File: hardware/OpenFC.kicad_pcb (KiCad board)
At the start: 6 copper layers, 27.6 x 27.6 mm, 135 parts, among them J10 5V, J12 5V, J14 5V, J15 5V, J17 5V, J18 5V, J20 5V, J21 5V, J22 5V, J24 5V, J25 5V, J26 5V, J27 5V, J28 5V, J29 5V, J30 5V, J31 5V, J32 5V, J33 5V, J34 5V, J35 5V, J37 5V, J39 5V, J40 5V, J41 5V, J42 5V, J43 5V, J44 5V, J45 5V, J46 5V, J48 5V, J49 5V, J5 5V, J8 5V, P1 SM08B-SRSS-TB(LF)(SN), Q5 AP1606, Q6 AP1606, U1 COS8051SOT, U10 RP2354A, U11 TS2306A 240GF MSM 9_C2976675, U18 SN74LVC1G3157DTBR, U2 TLV7031DPWR, U3 TI LMR51430YFDDCR, U4 TI LMR51430YFDDCR, U5 TPS2116DRLR, U6 NCV8187AMT180TAG, U7 LP5912-3.3DRVR, U8 SM06B-SRSS-TB(LF)(SN), U9 LSM6DSV16XTR, X1 XTM25012000JT00351001

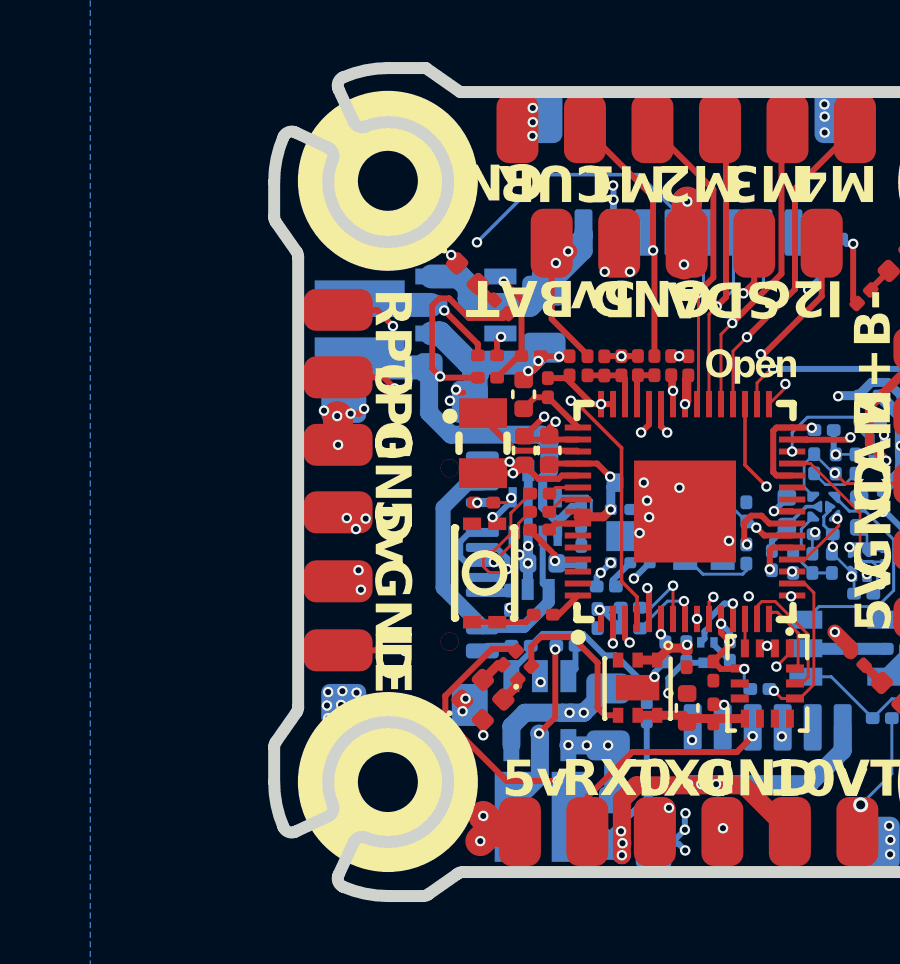
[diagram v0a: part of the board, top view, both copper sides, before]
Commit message: led names
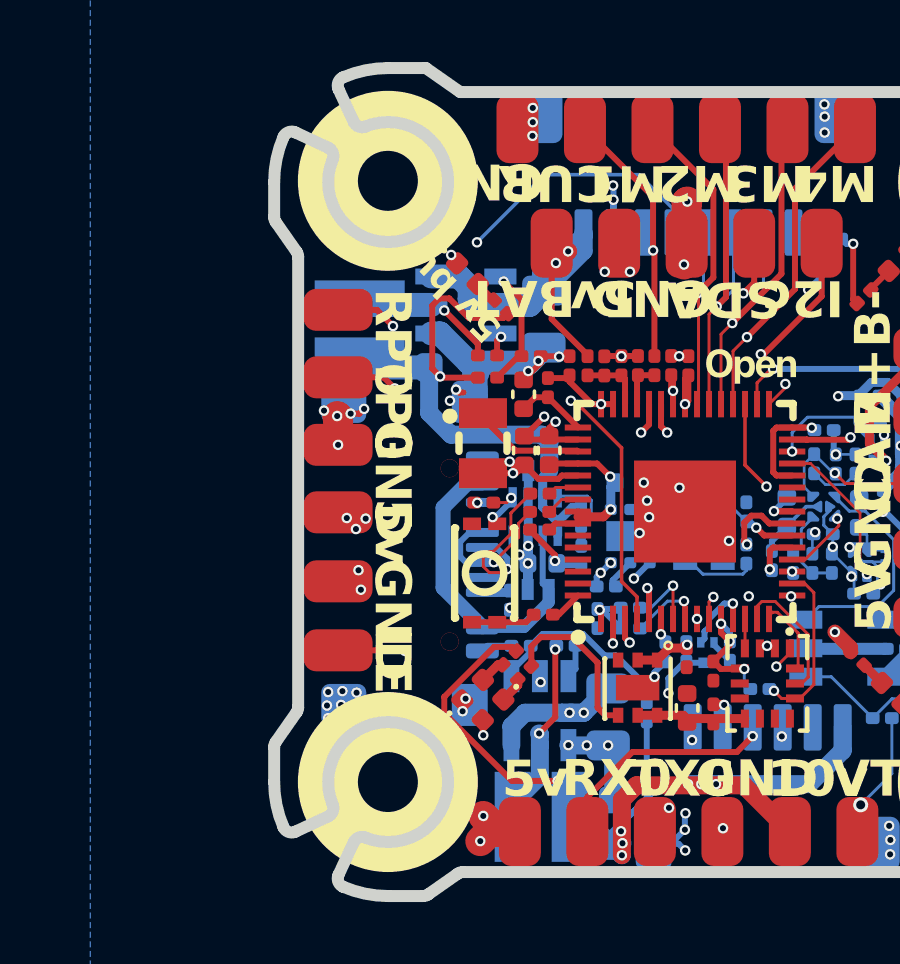
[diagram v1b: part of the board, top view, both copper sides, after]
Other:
- board text added: "10V+"
- board text added: "3v3+"
- board text added: "5v buck"
- board text added: "boot"
- board text added: "gyro"
- board text added: "status"

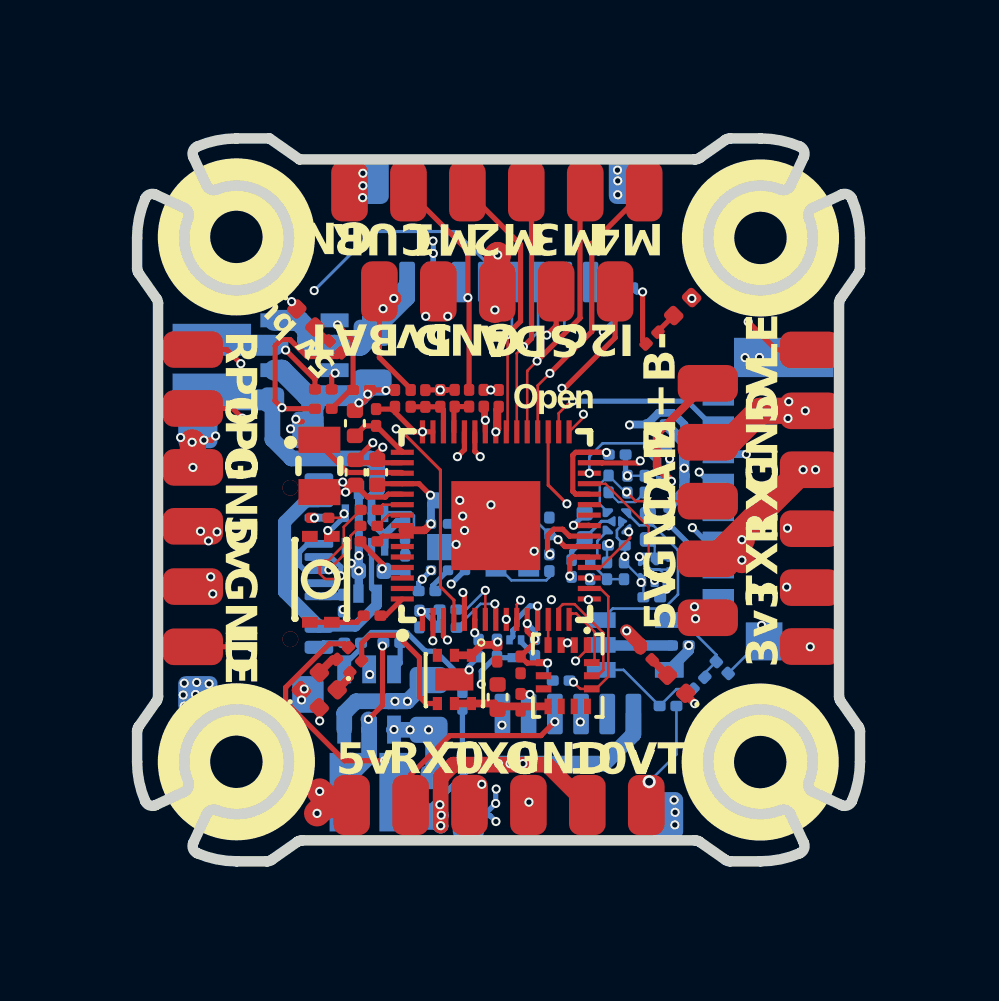
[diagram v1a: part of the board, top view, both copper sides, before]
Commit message: Clean routing
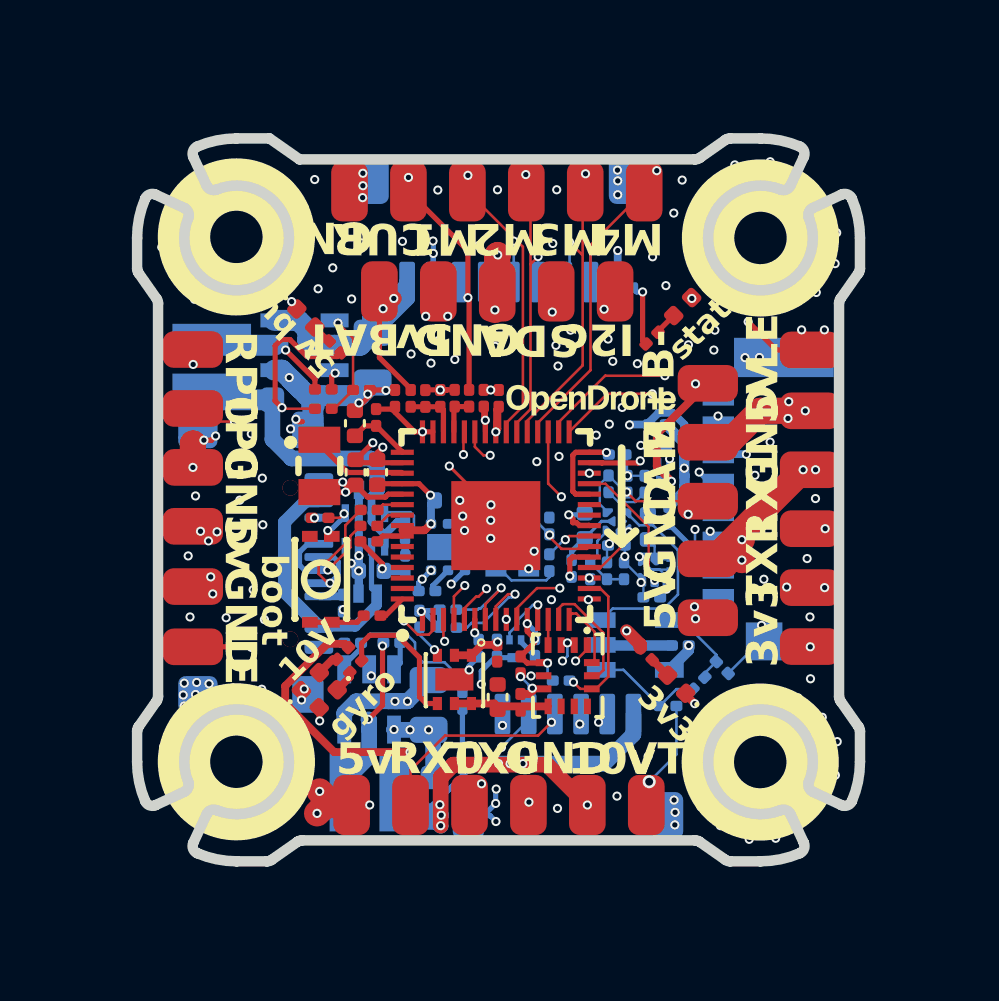
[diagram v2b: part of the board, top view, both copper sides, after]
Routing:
- net GND: track 84.7 -> 94.7 mm, vias 78 -> 182
- net /PADS/PIOUART0_TX: track 20.3 -> 14.7 mm
- net /PADS/LED_STRIP: track 53.4 -> 57.8 mm, vias 3 -> 5
- net /PADS/UART0_TX: track 13.6 -> 17.8 mm
- net /BLACKBOX/FLASH_CS: track 9.89 -> 13.7 mm
- net /PADS/U1RX: track 26.2 -> 29.3 mm
- net /POWER/10V_ENABLE: track 12.1 -> 14.9 mm
- net /PADS/UART0_RX: track 16.5 -> 14.1 mm
- net /PADS/M4: track 15.0 -> 12.5 mm, vias 1 -> 2
- net /BLACKBOX/SPI0.MOSI: track 8.15 -> 10.2 mm
- net /PADS/PU0RX: track 28.4 -> 30.1 mm
- net /PADS/M2: track 12.2 -> 10.8 mm, vias 1 -> 2
- net /PADS/M3: track 13.5 -> 12.4 mm, vias 1 -> 2
- net /RP2350A/LED0: track 12.5 -> 13.6 mm
- net /OSD/VIDEO_IN: track 5.90 -> 6.91 mm, vias 1 -> 2
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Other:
- board text added: "10V"
- board text removed: "10V+"
- board text removed: "3v3+"
